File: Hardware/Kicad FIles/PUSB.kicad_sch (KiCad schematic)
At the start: 31 parts, among them J1 Connector, USB-TYPE-C-16P, J5 2601-3104, J6 2601-3104, U1 AMS1117, U2 TPS5430DDAR, U3 AMS1117

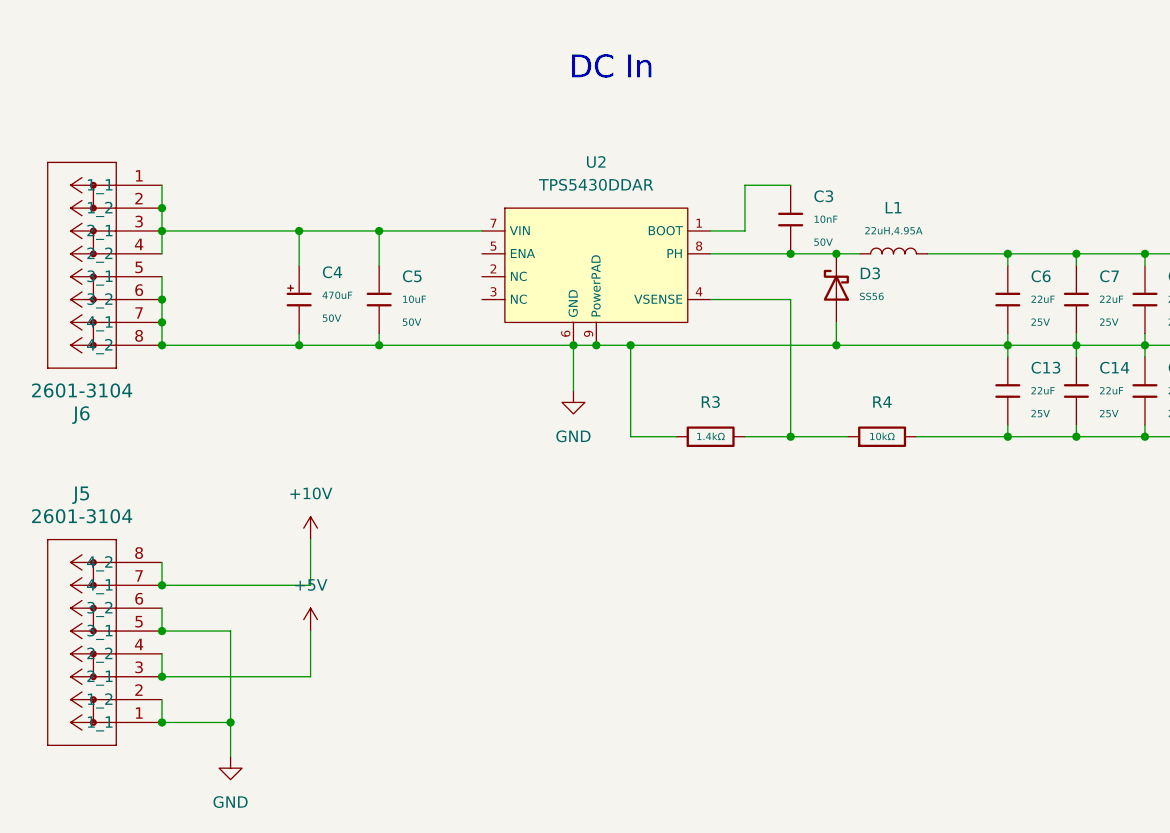
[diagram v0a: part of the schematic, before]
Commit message: Add files via upload
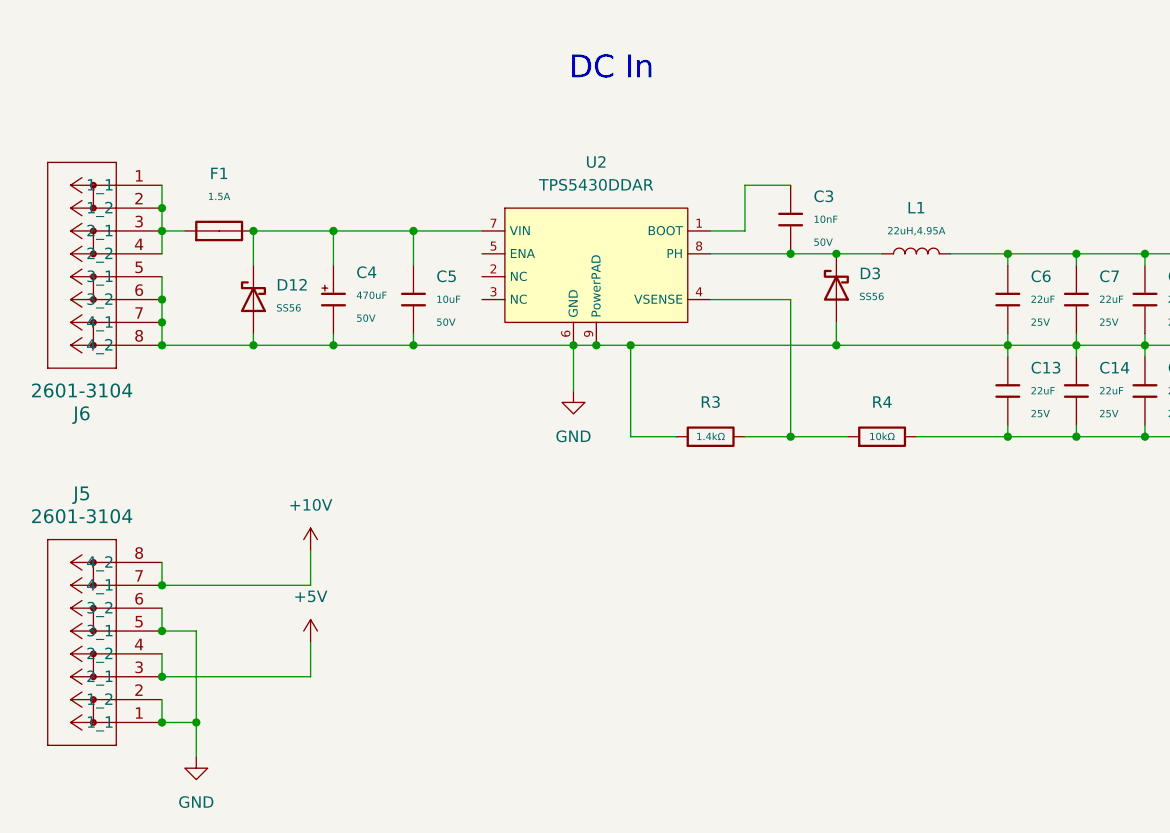
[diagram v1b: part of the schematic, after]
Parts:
- added D12: SS56, JLCPCB-Kicad-Footprints:D_SMC, symbol JLCPCB-Diodes:Schottky,SS56
- added F1: 1.5A, JLCPCB-Kicad-Footprints:F_1206, symbol JLCPCB-Variable-Resistors:Fuse,Resettable,1.5A
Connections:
- net GND: now also D12.2
- net at J6.1 (1_1), J6.2 (1_2), J6.3 (2_1)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: now also F1.1; no longer C4.1, C5.1, U2.7 (VIN)
- new net: C4.1, C5.1, D12.1, F1.2, U2.7 (VIN)
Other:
- moved on the sheet: C4, C5, L1
